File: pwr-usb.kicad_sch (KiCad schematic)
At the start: 18 parts, among them J1 Conn_01x16, J2 Conn_01x16, P1 USB_C_Plug_USB2.0, Q1 Q_PMOS_DGS, U4 NCP1117-3.3_SOT223

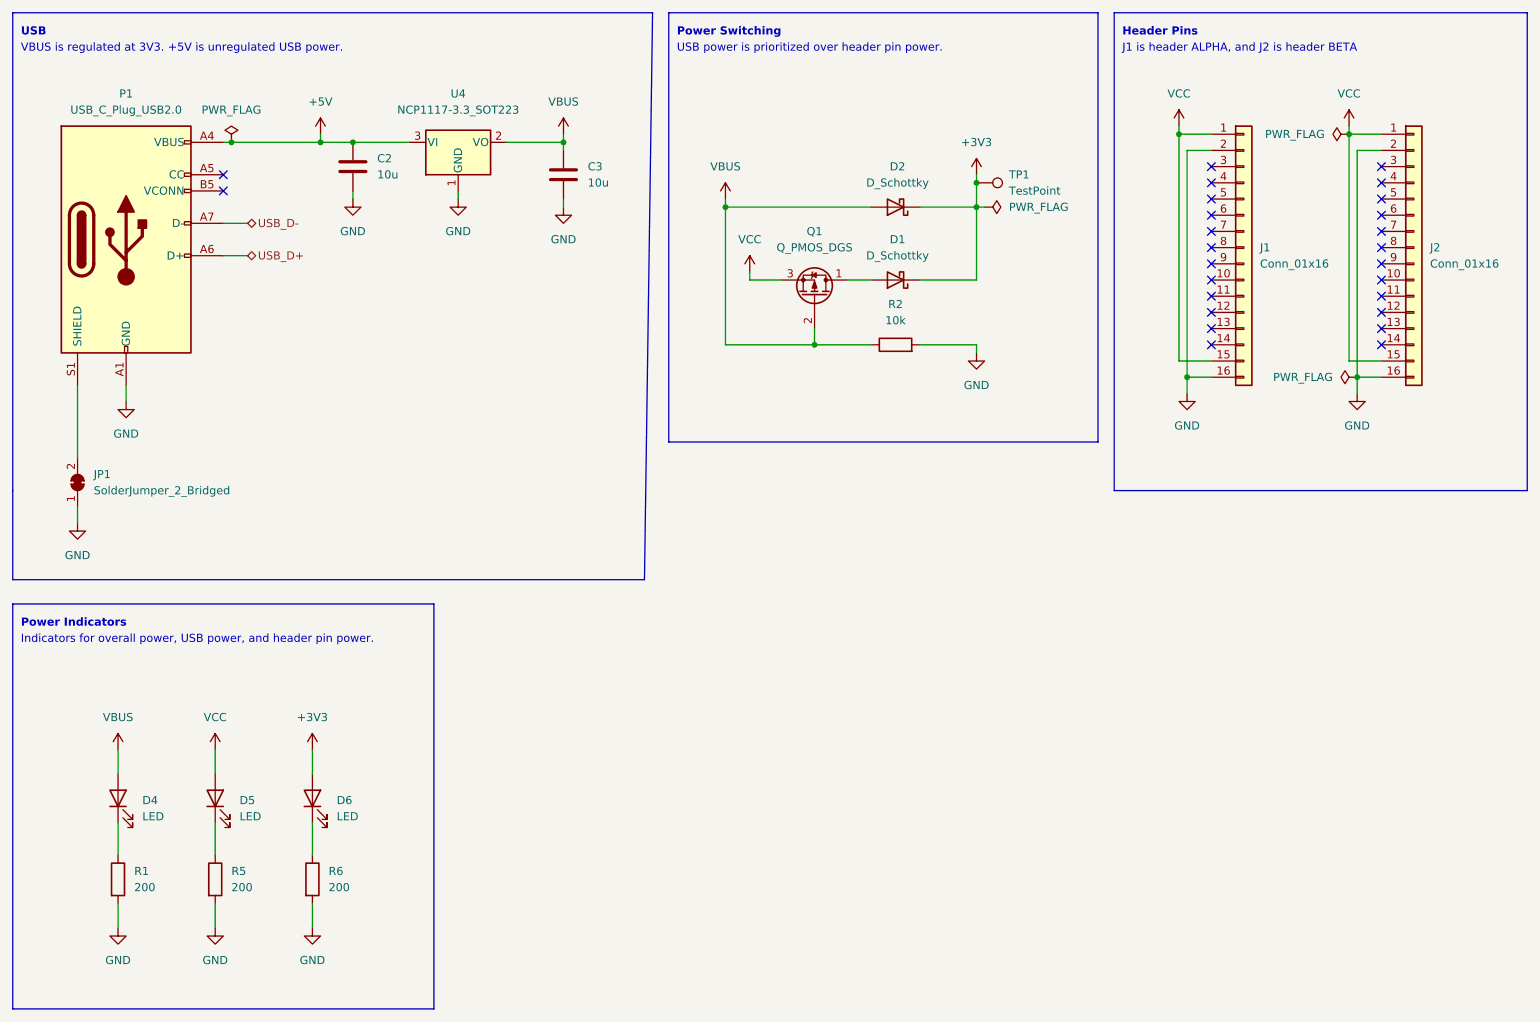
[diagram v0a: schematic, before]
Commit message: Fix many bugs with the initial version
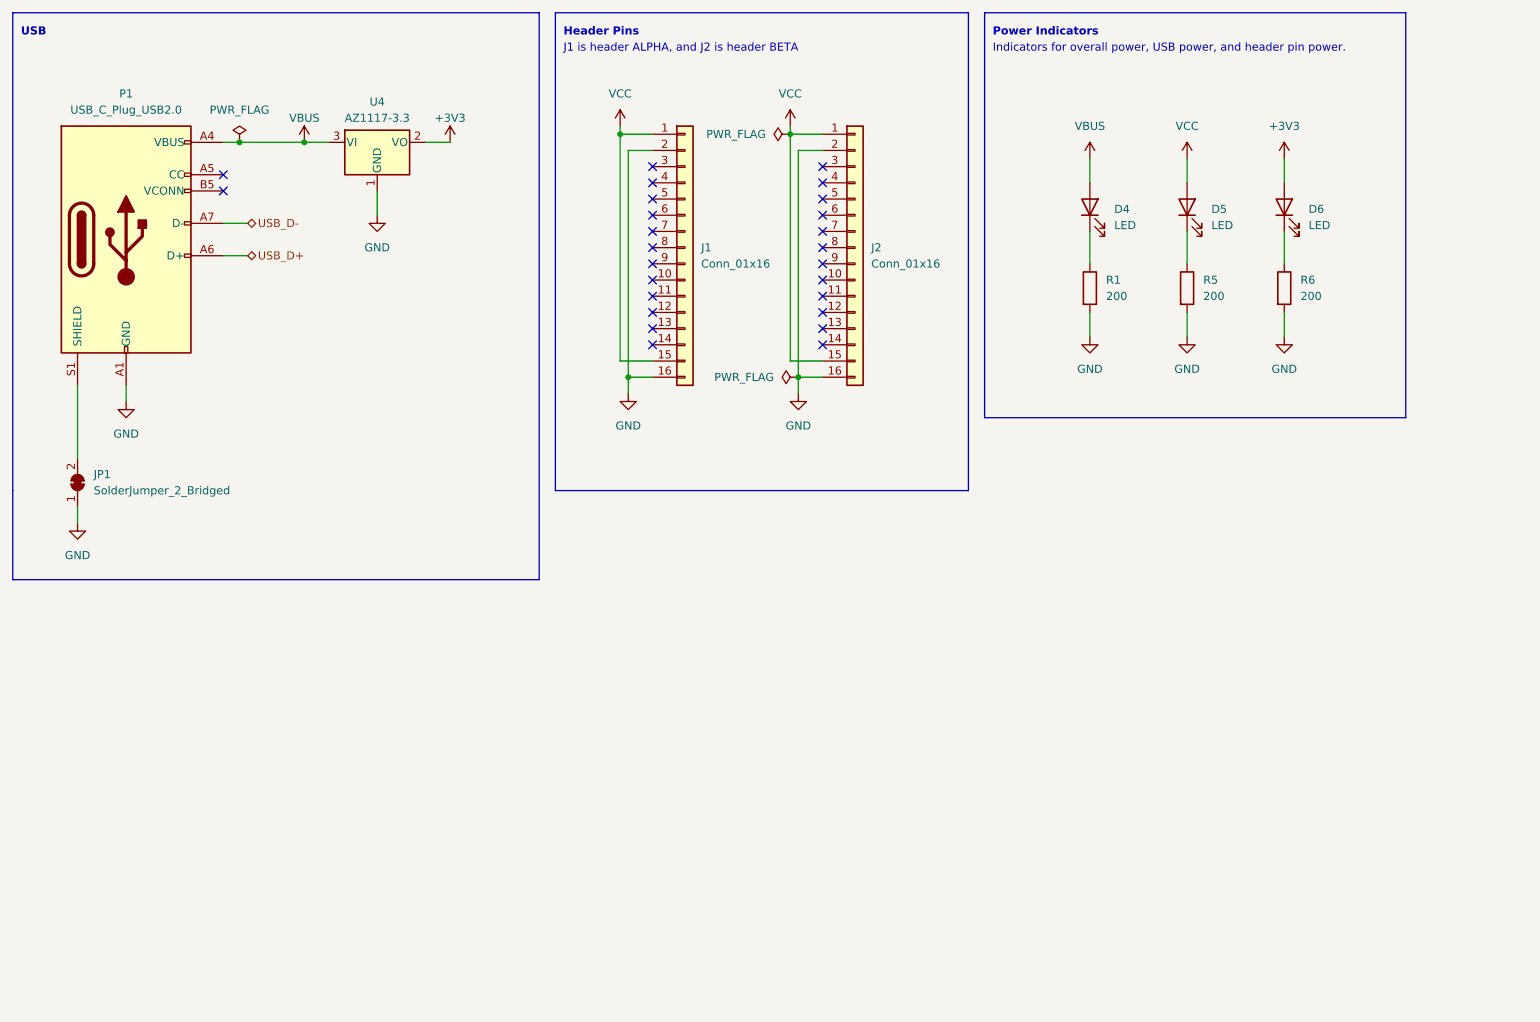
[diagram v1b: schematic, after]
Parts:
- removed C2, C3: 10u, Capacitor_SMD:C_1206_3216Metric_Pad1.33x1.80mm_HandSolder, symbol Device:C
- removed D1, D2: D_Schottky, Diode_SMD:D_SOD-323_HandSoldering, symbol Device:D_Schottky
- removed Q1: Q_PMOS_DGS, Package_TO_SOT_SMD:SC-59_Handsoldering, symbol Device:Q_PMOS_DGS
- removed R2: 10k, Resistor_SMD:R_0805_2012Metric_Pad1.20x1.40mm_HandSolder, symbol Device:R
- removed TP1: TestPoint, TestPoint:TestPoint_Loop_D2.54mm_Drill1.5mm_Beaded, symbol Connector:TestPoint
- removed U4: NCP1117-3.3_SOT223, Package_TO_SOT_SMD:SOT-223-3_TabPin2, symbol Regulator_Linear:NCP1117-3.3_SOT223
- added U4: AZ1117-3.3, Package_TO_SOT_SMD:SOT-223-3_TabPin2, symbol Regulator_Linear:AZ1117-3.3
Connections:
- net +5V is gone; now on net VBUS: P1.A4 (VBUS), P1.A9 (VBUS), P1.B4 (VBUS), P1.B9 (VBUS)
- net +3V3: now also U4.2 (VO)
- net GND: now also U4.1 (GND)
- net VBUS: now also U4.3 (VI)
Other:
- note removed: "Power Switching"
- note removed: "USB power is prioritized over header pin power."
- note removed: "VBUS is regulated at 3V3. +5V is unregulated USB power."
- moved on the sheet: D4, D5, D6, J1, J2, R1, R5, R6
